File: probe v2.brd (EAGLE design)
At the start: 11.8 x 29.5 mm, 12 parts, among them IC1 74AHC1G14DBV

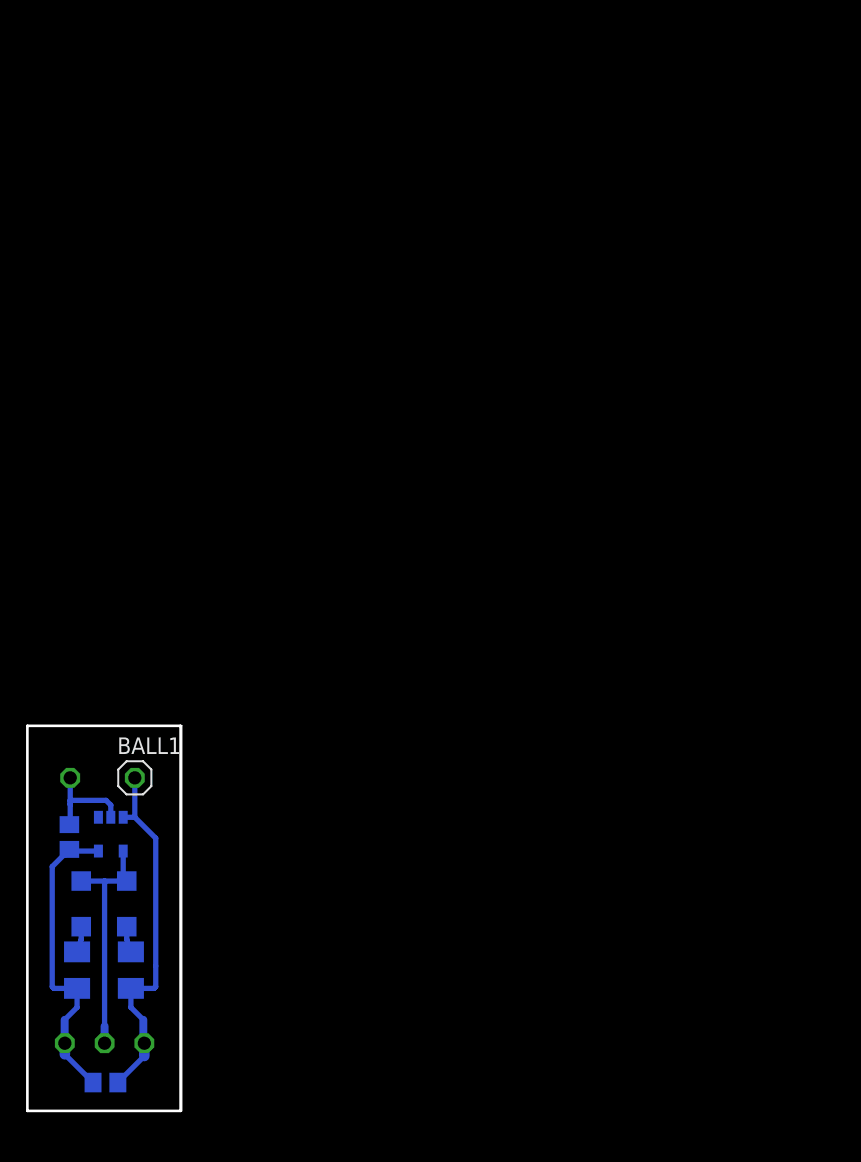
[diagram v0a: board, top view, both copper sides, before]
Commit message: First try to make a connection box directly on machine
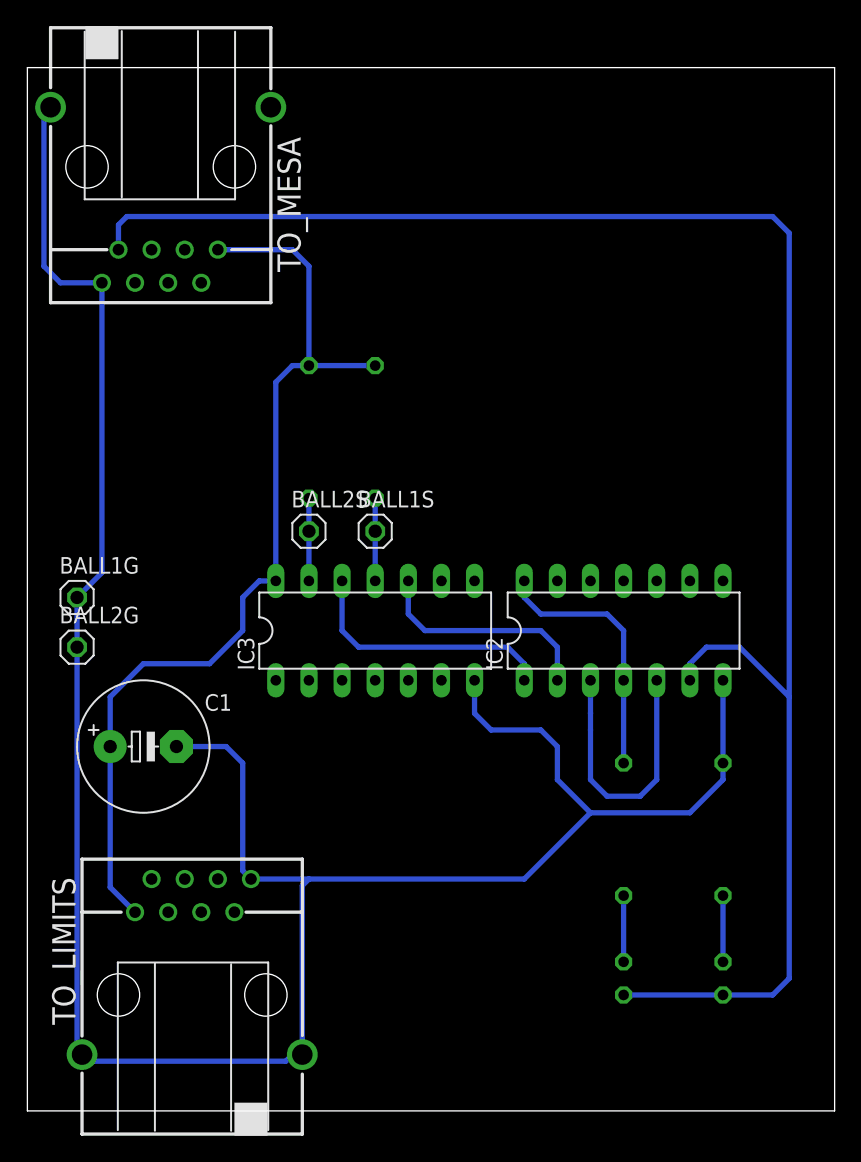
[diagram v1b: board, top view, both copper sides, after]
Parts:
- removed BALL, BALL1, GND, OUT, VCC: (no value), pinhead:1X01
- removed IC1: 74AHC1G14DBV, 74xx-little-us:SOT23-5
- added BALL1G, BALL1S, BALL2G, BALL2S: (no value), pinhead:1X01
- added IC2: 74AC00N, 74xx-eu:DIL14
- added IC3: 74AC14N, 74xx-eu:DIL14
- added R4: 1k, rcl:0207/10
- added TO_LIMITS, TO_MESA: (no value), con-amp:558310-1
- C1: device rcl:C0805 -> rcl:E5-10,5
- GREEN, RED: device led:CHIPLED_1206 -> led:LED5MM
- R1: device rcl:R0805 -> rcl:0207/10
- R2, R3: device rcl:M1206 -> rcl:0207/10
- moved R3 46.7 mm to (53.3, 21.6), turned to 270 degrees
- moved RED 46.1 mm to (53.3, 10.2), turned to 90 degrees
- moved R2 43.3 mm to (45.7, 21.6), turned to 90 degrees
- moved GREEN 42.0 mm to (45.7, 10.2), turned to 270 degrees
- moved R1 38.9 mm to (26.7, 52.1), turned to 90 degrees
- moved C1 25.9 mm to (8.89, 27.9), flipped to the top, turned to 0 degrees
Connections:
- removed net OUT: GREEN.C, IC1.4, OUT.1, RED.A
- new net LIMIT_A: TO_MESA.5
- new net LIMIT_X: TO_MESA.2
- new net LIMIT_Y: TO_MESA.3
- new net LIMIT_Z: TO_MESA.4
- new net N$12: TO_MESA.6
- new net N$4: IC2.1, IC3.12
- new net N$5: IC2.2, IC3.10
- new net N$6: BALL2S.1, IC3.13, R4.1
- new net N$7: IC2.3, IC2.5
- new net PROBE: GREEN.K, IC2.6, RED.A, TO_MESA.7
- net BALL: now also BALL1S.1, IC3.11; no longer BALL.1, IC1.2
- net GND: now also BALL1G.1, BALL2G.1, C1.-, IC2.7, IC3.7, TO_LIMITS.8, TO_LIMITS.G2, TO_MESA.8, TO_MESA.G2; no longer BALL1.1, C1.2, GND.1, IC1.3
- net N$2: now also RED.K; no longer RED.C
- net VCC: now also C1.+, IC2.14, IC2.4, IC3.14, R4.2, TO_LIMITS.1, TO_MESA.1; no longer C1.1, IC1.5, VCC.1
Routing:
- net GND: track 28.2 -> 187.1 mm
- net PROBE: track 0.00 -> 135.5 mm
- net VCC: track 23.8 -> 93.8 mm
- net N$7: track 0.00 -> 21.4 mm
- net N$4: track 0.00 -> 20.1 mm
- net OUT: track 18.5 -> 0.00 mm
- net N$5: track 0.00 -> 17.6 mm
- net N$6: track 0.00 -> 6.35 mm
- net N$2: track 1.98 -> 5.08 mm
- net N$1: track 1.98 -> 5.08 mm
- net BALL: track 8.16 -> 6.35 mm
- net N$3: track 1.30 -> 0.00 mm
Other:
- board size 11.8 x 29.5 mm -> 61.9 x 80 mm
